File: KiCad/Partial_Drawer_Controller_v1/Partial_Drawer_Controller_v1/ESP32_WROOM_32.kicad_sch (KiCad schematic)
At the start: 37 parts, among them Q1 SS8050, Q2 2N7002T-7-F, Q3 2N7002T-7-F, Q5 SS8050, U6 CP2102N-Axx-xQFN28, U7 ESP32-WROOM-32E_8N, X1 USB-Micro

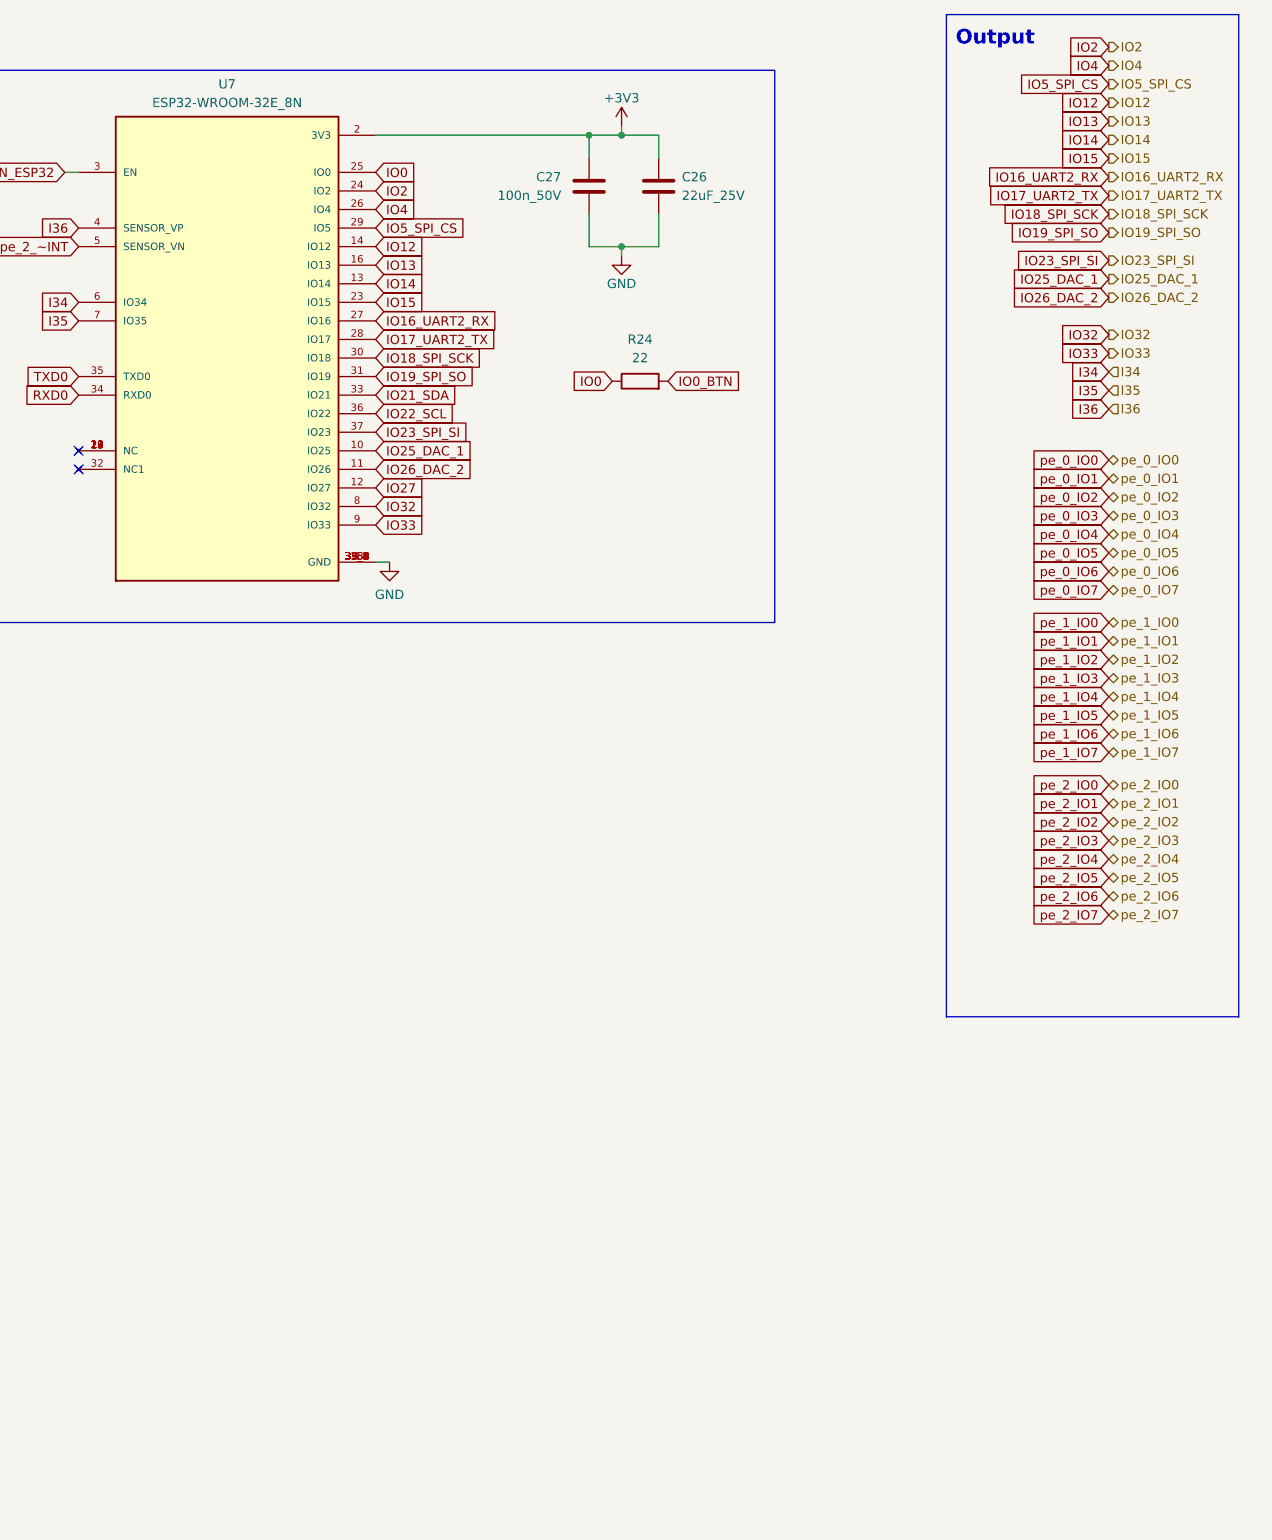
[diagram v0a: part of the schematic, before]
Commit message: feat: some small progress
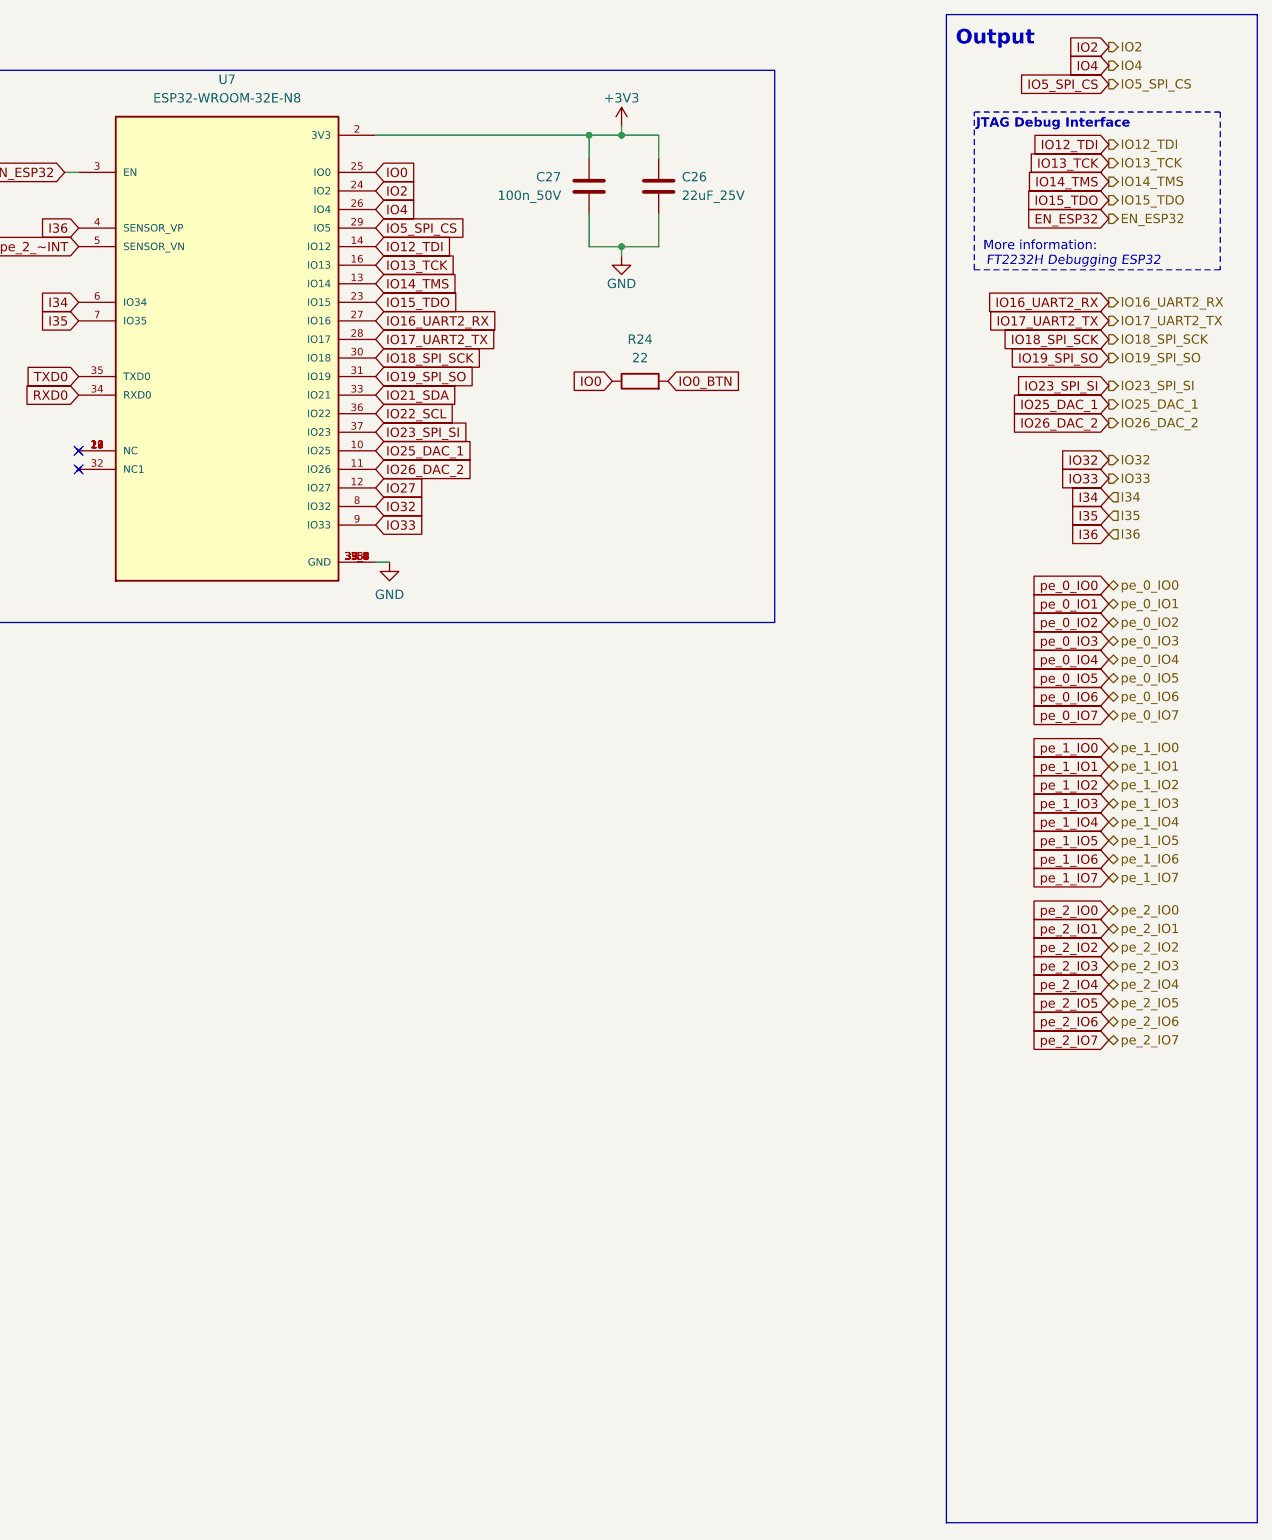
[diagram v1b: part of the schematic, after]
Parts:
- removed U7: ESP32-WROOM-32E_8N, Robast_Footprints:XCVR_ESP32-WROOM-32E_(16MB), symbol ESP32-WROOM-32E__16MB_:ESP32-WROOM-32E_(16MB)
- added U7: ESP32-WROOM-32E-N8, Robast:ESP32-WROOM-32E, symbol _MCU:ESP32-WROOM-32E-N8
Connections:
- net +3V3: now also U7.2 (3V3)
- net EN_ESP32: now also U7.3 (EN)
- net GND: now also U7.1 (GND), U7.15 (GND), U7.38 (GND), U7.39_1 (GND), U7.39_2 (GND), U7.39_3 (GND), U7.39_4 (GND), U7.39_5 (GND), U7.39_6 (GND), U7.39_7 (GND), U7.39_8 (GND), U7.39_9 (GND)
- net I34: now also U7.6 (IO34)
- net I35: now also U7.7 (IO35)
- net I36: now also U7.4 (SENSOR_VP)
- net IO0: now also U7.25 (IO0)
- net IO16_UART2_RX: now also U7.27 (IO16)
- net IO17_UART2_TX: now also U7.28 (IO17)
- net IO18_SPI_SCK: now also U7.30 (IO18)
- net IO19_SPI_SO: now also U7.31 (IO19)
- net IO2: now also U7.24 (IO2)
- net IO21_SDA: now also U7.33 (IO21)
- net IO22_SCL: now also U7.36 (IO22)
- net IO23_SPI_SI: now also U7.37 (IO23)
- net IO25_DAC_1: now also U7.10 (IO25)
- net IO26_DAC_2: now also U7.11 (IO26)
- net IO27: now also U7.12 (IO27)
- net IO32: now also U7.8 (IO32)
- net IO33: now also U7.9 (IO33)
- net IO4: now also U7.26 (IO4)
- net IO5_SPI_CS: now also U7.29 (IO5)
- net RXD0: now also U7.34 (RXD0)
- net TXD0: now also U7.35 (TXD0)
- net pe_2_~INT: now also U7.5 (SENSOR_VN)
- new net: U7.17 (NC), U7.18 (NC), U7.19 (NC), U7.20 (NC), U7.21 (NC), U7.22 (NC)
- new net IO12_TDI: U7.14 (IO12)
- new net IO13_TCK: U7.16 (IO13)
- new net IO14_TMS: U7.13 (IO14)
- new net IO15_TDO: U7.23 (IO15)
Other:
- note added: "FT2232H Debugging ESP32"
- note added: "JTAG Debug Interface"
- note added: "More information:"
